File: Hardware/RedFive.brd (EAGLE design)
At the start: 68.6 x 53.3 mm, 131 parts, among them IC3 LM1117, J2 USB Female Type C Connector, J3 POWER_JACKSUPER_BOMB_DIGITY, J5 CORTEX_JTAG_DEBUG_SMD, Q1 1.1A/60V/600mΩ, U1 CH340C, U2 1.8V, U3 AP2112-3.3V, U4 FE310, U5 32MB, Y1 32.768KHZ, Y2 16MHz

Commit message: Adding prod_id to JTAG
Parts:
- J5: value CORTEX_JTAG_DEBUG_SMD -> JTAG
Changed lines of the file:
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@@
 <element name="F1" library="SparkFun-Fuses" package="0805" value="6V 0.5A" x="6.35" y="29.845" smashed="yes">
 <attribute name="NAME" x="6.35" y="30.734" size="0.6096" layer="25" font="vector" ratio="20" align="bottom-center"/>
-<attribute name="PROD_ID" value="13945" x="6.35" y="29.845" size="1.778" layer="27" display="off"/>
+<attribute name="PROD_ID" value="RES-13945" x="6.35" y="29.845" size="1.778" layer="27" display="off"/>
 <attribute name="VALUE" x="6.35" y="28.956" size="0.6096" layer="27" font="vector" ratio="20" align="top-center"/>
 </element>
@@
 <attribute name="PROD_ID" value="IC-14494" x="41.91" y="34.29" size="1.778" layer="27" display="off"/>
 </element>
-<element name="J5" library="SparkFun-Connectors" package="2X5-SMD-1.27MM" value="CORTEX_JTAG_DEBUG_SMD" x="43.18" y="17.78" smashed="yes" rot="R180"/>
+<element name="J5" library="SparkFun-Connectors" package="2X5-SMD-1.27MM" value="JTAG" x="43.18" y="17.78" smashed="yes" rot="R180">
+<attribute name="PROD_ID" value="CONN-14503" x="43.18" y="17.78" size="1.778" layer="27" rot="R180" display="off"/>
+<attribute name="VALUE" value="JTAG" x="43.18" y="17.78" size="1.778" layer="27" rot="R180" display="off"/>
+</element>
 <element name="C1" library="SparkFun-Capacitors" package="0603" value="10uF" x="49.53" y="38.354" smashed="yes">
 <attribute name="NAME" x="49.53" y="39.116" size="0.6096" layer="25" font="vector" ratio="20" align="bottom-center"/>

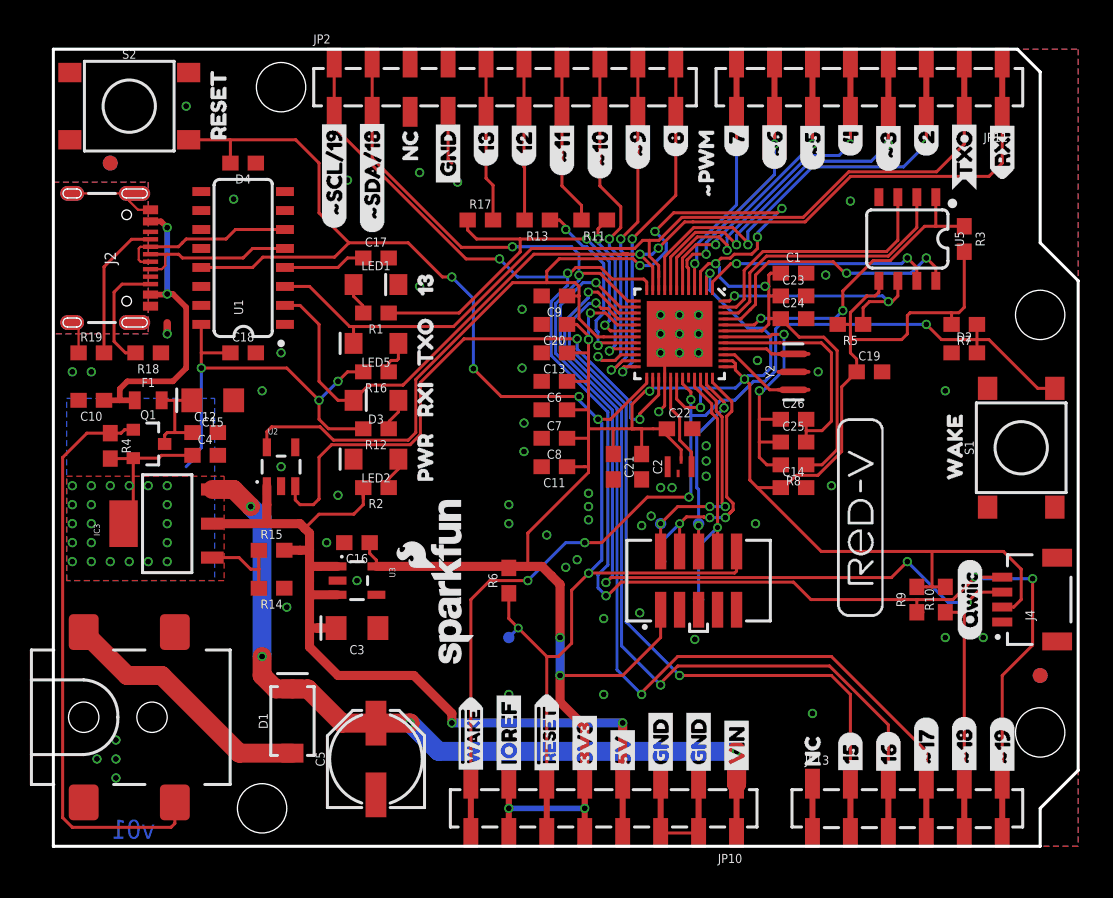
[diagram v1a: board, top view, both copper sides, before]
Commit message: v02
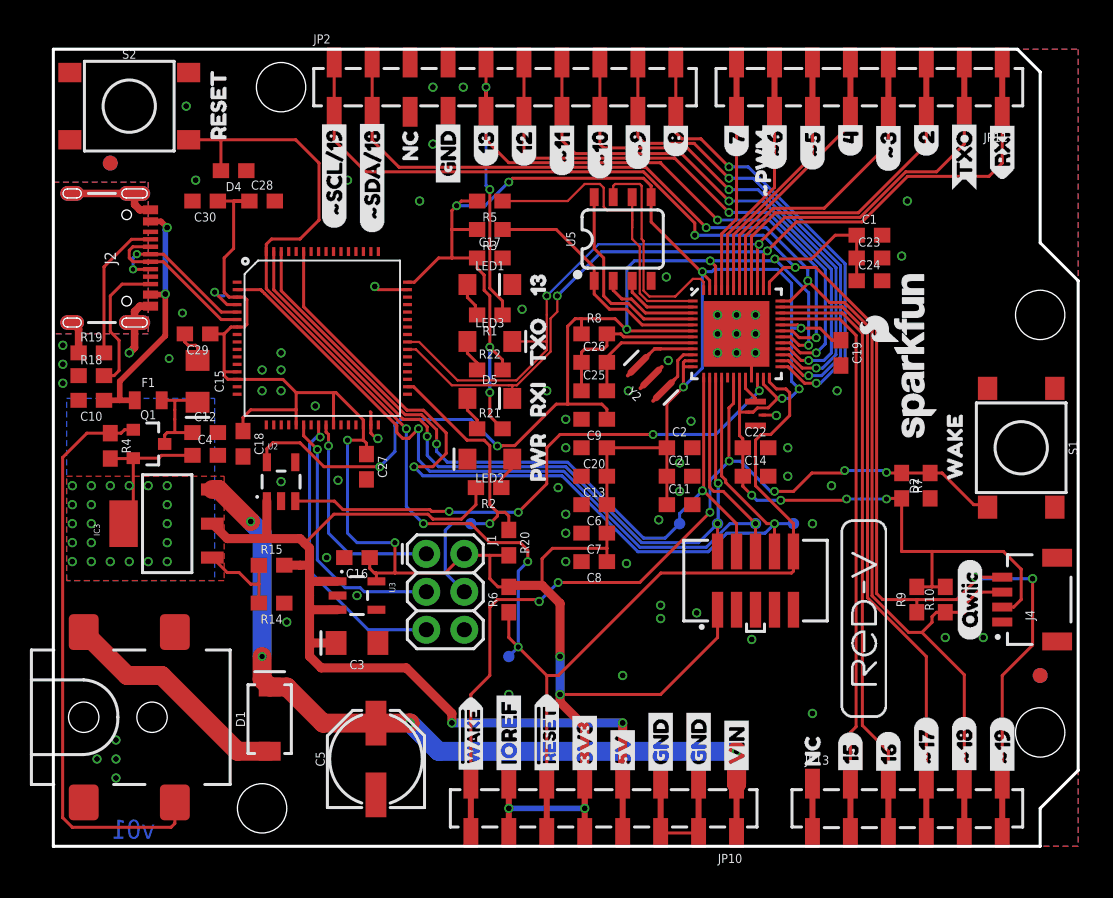
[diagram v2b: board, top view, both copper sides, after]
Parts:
- removed D3: YELLOW, SparkFun-LED:LED-1206-HIDDENSILK
- removed LED5: GREEN, SparkFun-LED:LED-1206
- removed R11, R13, R17: 22, SparkFun-Resistors:0603
- removed R12, R16: 4.7k, SparkFun-Resistors:0603
- removed U1: CH340C, SparkFun-IC-Comms:SO016
- added C27, C28, C29: 0.1uF, SparkFun-Capacitors:0603
- added C30: 10uF, SparkFun-Capacitors:0603
- added D5: YELLOW, SparkFun-LED:LED-1206-HIDDENSILK
- added J1: AVR_SPI_PROG_3X2PTH, SparkFun-Connectors:2X3
- added LED3: GREEN, SparkFun-LED:LED-1206
- added R20: 100k, SparkFun-Resistors:0603
- added R21, R22: 4.7k, SparkFun-Resistors:0603
- added TP6, TP7, TP8: TEST-POINT3, SparkFun-Connectors:PAD.03X.03
- added U$44: MK22FN128VLH10, SparkFun-IC-Comms:LQFP-64
- C17: value 10nF -> 0.1uF
- moved LOGO1 34.5 mm to (57.7, 32.9)
- moved R3 31.8 mm to (29.2, 41.3), turned to 180 degrees
- moved R5 25.5 mm to (29.2, 43.2)
- moved U5 19.0 mm to (38.1, 40.6), turned to 0 degrees
- moved R8 16.0 mm to (36.2, 34.3), turned to 0 degrees
- moved C26 13.9 mm to (36.2, 32.4)
- moved C25 13.8 mm to (36.2, 30.5)
- moved R7 11.6 mm to (56.8, 24.1), turned to 270 degrees
- moved Y2 9.53 mm to (40.0, 31.4), turned to 135 degrees
- moved D2 9.18 mm to (58.7, 24.1), turned to 90 degrees
- moved C11 8.76 mm to (41.9, 22.9), turned to 0 degrees
- moved C13 8.68 mm to (36.2, 24.8)
- moved C7 8.68 mm to (36.2, 21.0)
- moved C6 8.68 mm to (36.2, 22.9)
- moved C8 8.68 mm to (36.2, 19.1)
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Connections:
- removed net N$11: JP2.7A, JP2.7B, R11.2
- removed net N$14: J2.A6, J2.B6, U1.5
- removed net N$16: JP2.5A, JP2.5B, R17.2
- removed net N$4: JP2.6A, JP2.6B, R13.2
- removed net N$5: LED5.A, R16.1
- removed net N$9: D3.A, R12.1
- new net D+: J2.A6, J2.B6, U$44.5
- new net D-: J2.A7, J2.B7, U$44.6
- new net DBG_RESET: J1.4, R20.1, TP8.P$1, U$44.34
- new net DBG_SWDCLK: J1.3, U$44.22
- new net DBG_SWDIO: J1.1, U$44.25
- new net DBG_SWO: J1.5, U$44.24
- net !RESET: now also U$44.64; no longer U1.13
- net 3.3V: now also C17.1, C18.1, C27.1, C28.1, C29.1, C30.1, J1.2, R20.2, R21.2, R22.2, TP6.P$1, U$44.13, U$44.14, U$44.21, U$44.26, U$44.3, U$44.30, U$44.48, U$44.7
- net 5V: no longer C18.1, R12.2, R16.2, U1.16
- net GND: now also C27.2, C28.2, C29.2, C30.2, J1.6, TP7.P$1, U$44.15, U$44.16, U$44.31, U$44.4, U$44.47; no longer U1.1
- net N$13: now also D5.A, R21.1; no longer J2.A7, J2.B7, U1.6
- net N$6: now also LED3.A, R22.1; no longer C17.1, U1.4
- net RXI: now also D5.C, U$44.39; no longer D3.C, U1.2
- net SPI_MISO: now also JP2.6A, JP2.6B; no longer R13.1
- net SPI_MOSI: now also JP2.7A, JP2.7B; no longer R11.1
- net SPI_SCK: now also JP2.5A, JP2.5B; no longer R17.1
- net TCK: now also U$44.62
- net TDI: now also U$44.59
- net TDO: now also U$44.2
- net TMS: now also U$44.63
- net TXO: now also LED3.C, U$44.40; no longer LED5.C, U1.3
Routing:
- net 3.3V: track 193.0 -> 263.0 mm, vias 10 -> 19
- net TDI: track 17.6 -> 62.6 mm, vias 1 -> 2
- net TDO: track 13.1 -> 57.8 mm
- net TMS: track 16.0 -> 52.6 mm
- net TCK: track 19.4 -> 52.9 mm, vias 3 -> 2
- net SPI_SCK: track 29.0 -> 55.5 mm, vias 2 -> 4
- net SPI_MOSI: track 11.5 -> 37.0 mm
- net SPI_MISO: track 13.3 -> 38.0 mm
- net IO11: track 62.9 -> 38.4 mm, vias 2 -> 0
- net DBG_RESET: track 0.00 -> 22.4 mm, vias 0 -> 1
- net 5V: track 101.1 -> 78.9 mm, vias 26 -> 23
- net DBG_SWO: track 0.00 -> 19.8 mm, vias 0 -> 1
- net IO9: track 53.3 -> 35.7 mm, vias 2 -> 0
- net IO10: track 58.1 -> 40.4 mm, vias 2 -> 0
- net DBG_SWDCLK: track 0.00 -> 17.6 mm, vias 0 -> 1
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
